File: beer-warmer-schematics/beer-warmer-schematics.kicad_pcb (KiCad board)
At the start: 4 copper layers, 60 x 42.8 mm, 29 parts, among them J1 USB_C_Receptacle_USB2.0_14P, J2 Screw_Terminal_01x02, J3 Conn_01x07_Socket, J4 Conn_01x07_Socket, J5 Conn_01x04_Pin, J6 Screw_Terminal_01x03, Q1 AOD4184A, U2 LM2596S-5, U3 CH224K

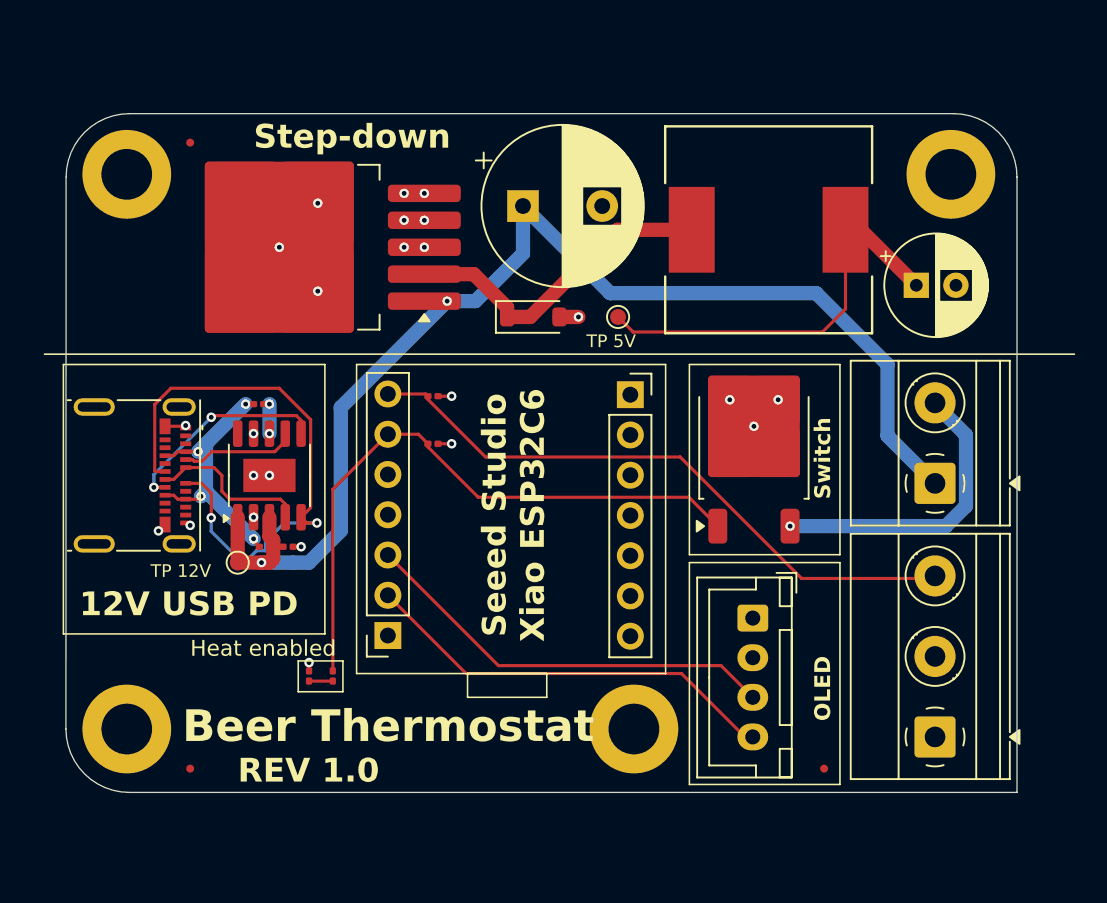
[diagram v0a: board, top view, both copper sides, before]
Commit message: cleanup
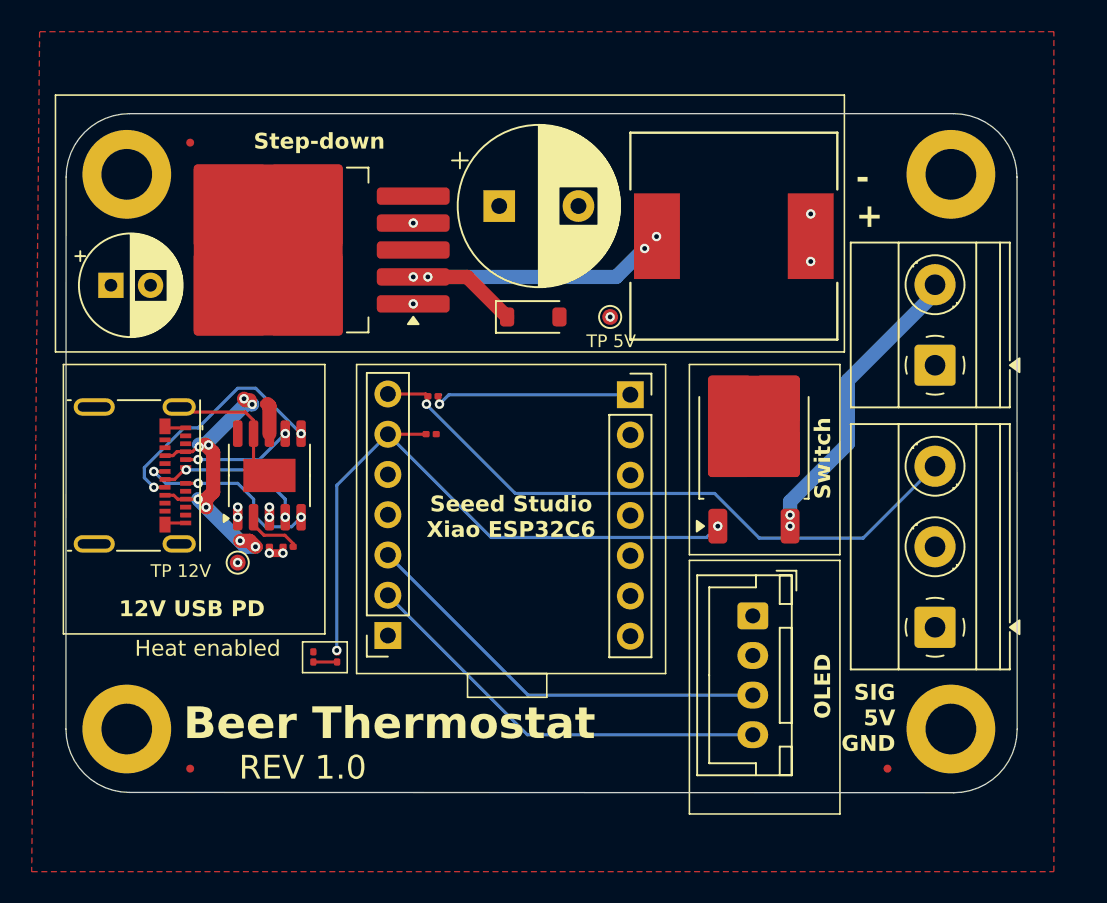
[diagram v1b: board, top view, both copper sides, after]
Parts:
- moved C3 50.8 mm to (122.5, 82.0)
- moved H4 20.0 mm to (175.5, 110.0)
- moved J2 7.45 mm to (174.5, 87.0)
- moved J6 6.92 mm to (174.5, 103.6)
- moved FID3 4.00 mm to (171.5, 112.5)
- moved L1 2.23 mm to (161.8, 78.9)
- moved C2 1.50 mm to (147.0, 77.0)
- moved D2 1.23 mm to (135.3, 105.5)
- moved R3 1.23 mm to (136.8, 105.5)
- moved U2 0.72 mm to (133.9, 79.8)
- moved R2 0.62 mm to (142.7, 91.4)
- moved TP2 0.50 mm to (154.0, 84.0)
- moved J5 0.14 mm to (163.0, 102.9)
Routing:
- net VDD: track 76.3 -> 1.59 mm, vias 2 -> 8
- net Net-(U3-DM): track 36.4 -> 13.1 mm, vias 2 -> 3
- net +5V: track 27.1 -> 12.9 mm, vias 3 -> 5
- net GND: track 5.33 -> 15.3 mm, vias 21 -> 0
- net Net-(J1-VBUS-PadA4): track 17.7 -> 21.2 mm, vias 4 -> 8
- net Net-(J1-CC2): track 13.3 -> 15.4 mm
- net Net-(D1-K): track 20.6 -> 22.5 mm, vias 0 -> 4
- net D1: track 39.7 -> 41.2 mm, vias 0 -> 2
- net D0: track 39.5 -> 40.6 mm, vias 0 -> 1
- net Net-(U3-DP): track 10.3 -> 9.74 mm, vias 0 -> 2
- net Net-(J2-Pin_2): track 18.9 -> 18.5 mm, vias 1 -> 2
- net Net-(J1-CC1): track 7.33 -> 6.96 mm, vias 0 -> 2
- net Net-(U3-VBUS): track 2.22 -> 1.91 mm, vias 2 -> 0
- added copper zone on In1.Cu, net +5V
- added copper zone on F.Cu, net GND
- added copper zone on In2.Cu, net VDD
- removed copper zone on In2.Cu, net +5V
- removed copper zone on In1.Cu, net GND
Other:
- outline, holes or cut-outs redrawn
- board text added: "- +"
